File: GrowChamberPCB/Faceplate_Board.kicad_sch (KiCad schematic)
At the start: 4 parts, among them J10 Conn_01x24_Pin, J6 Conn_01x04_Pin

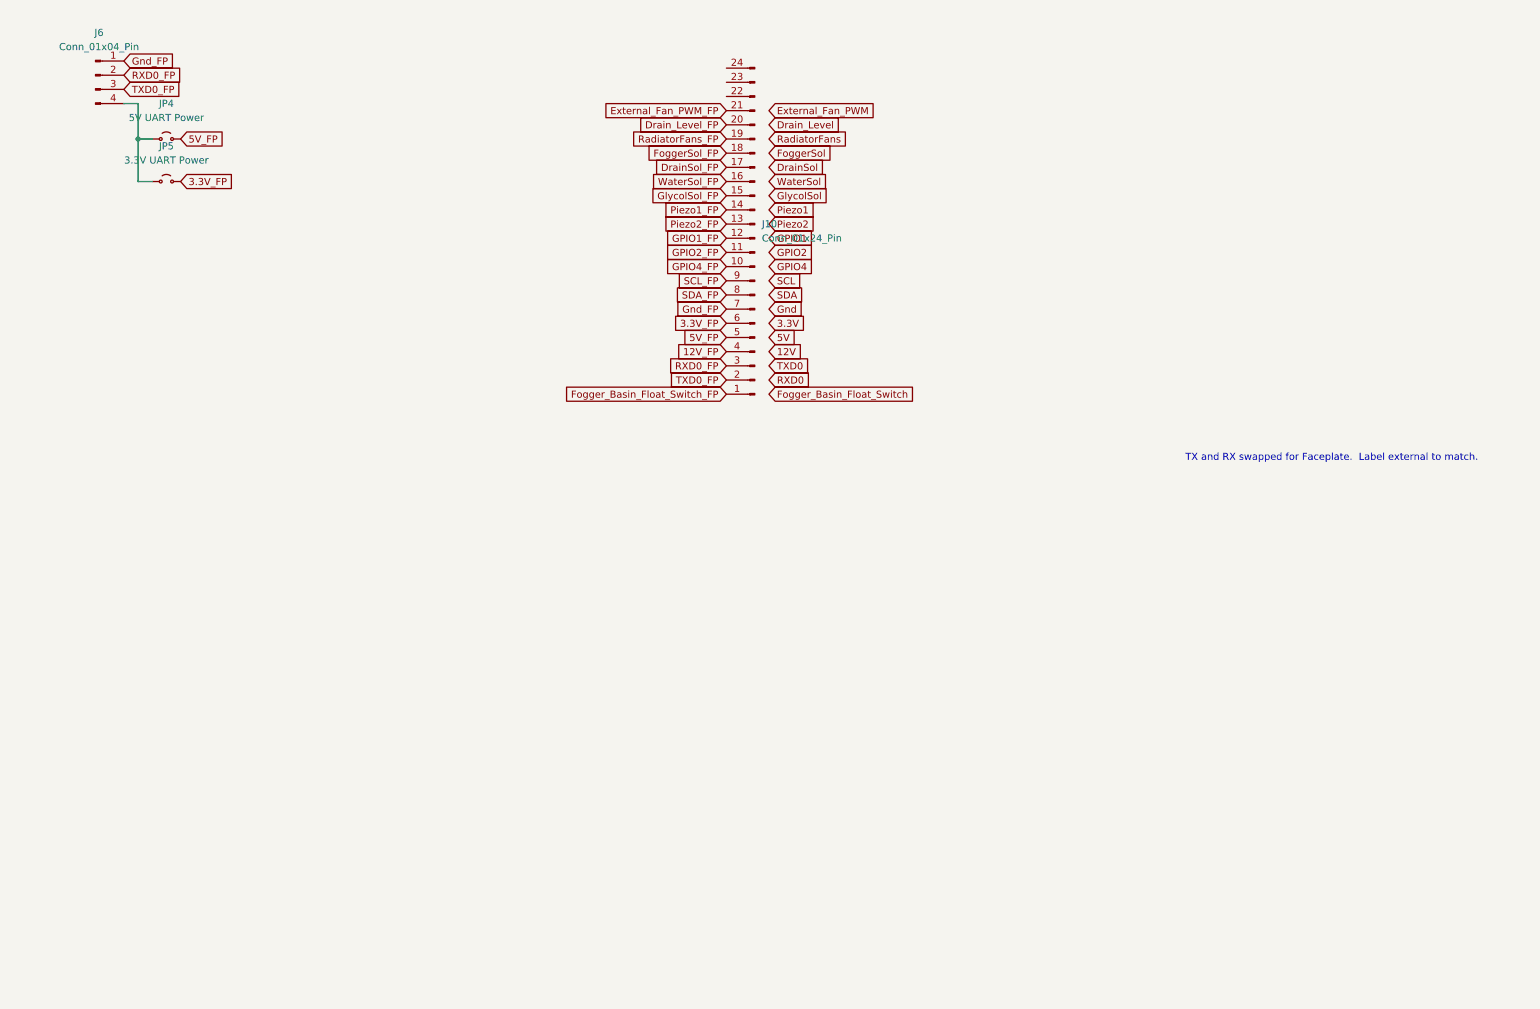
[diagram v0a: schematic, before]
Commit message: Working on faceplate
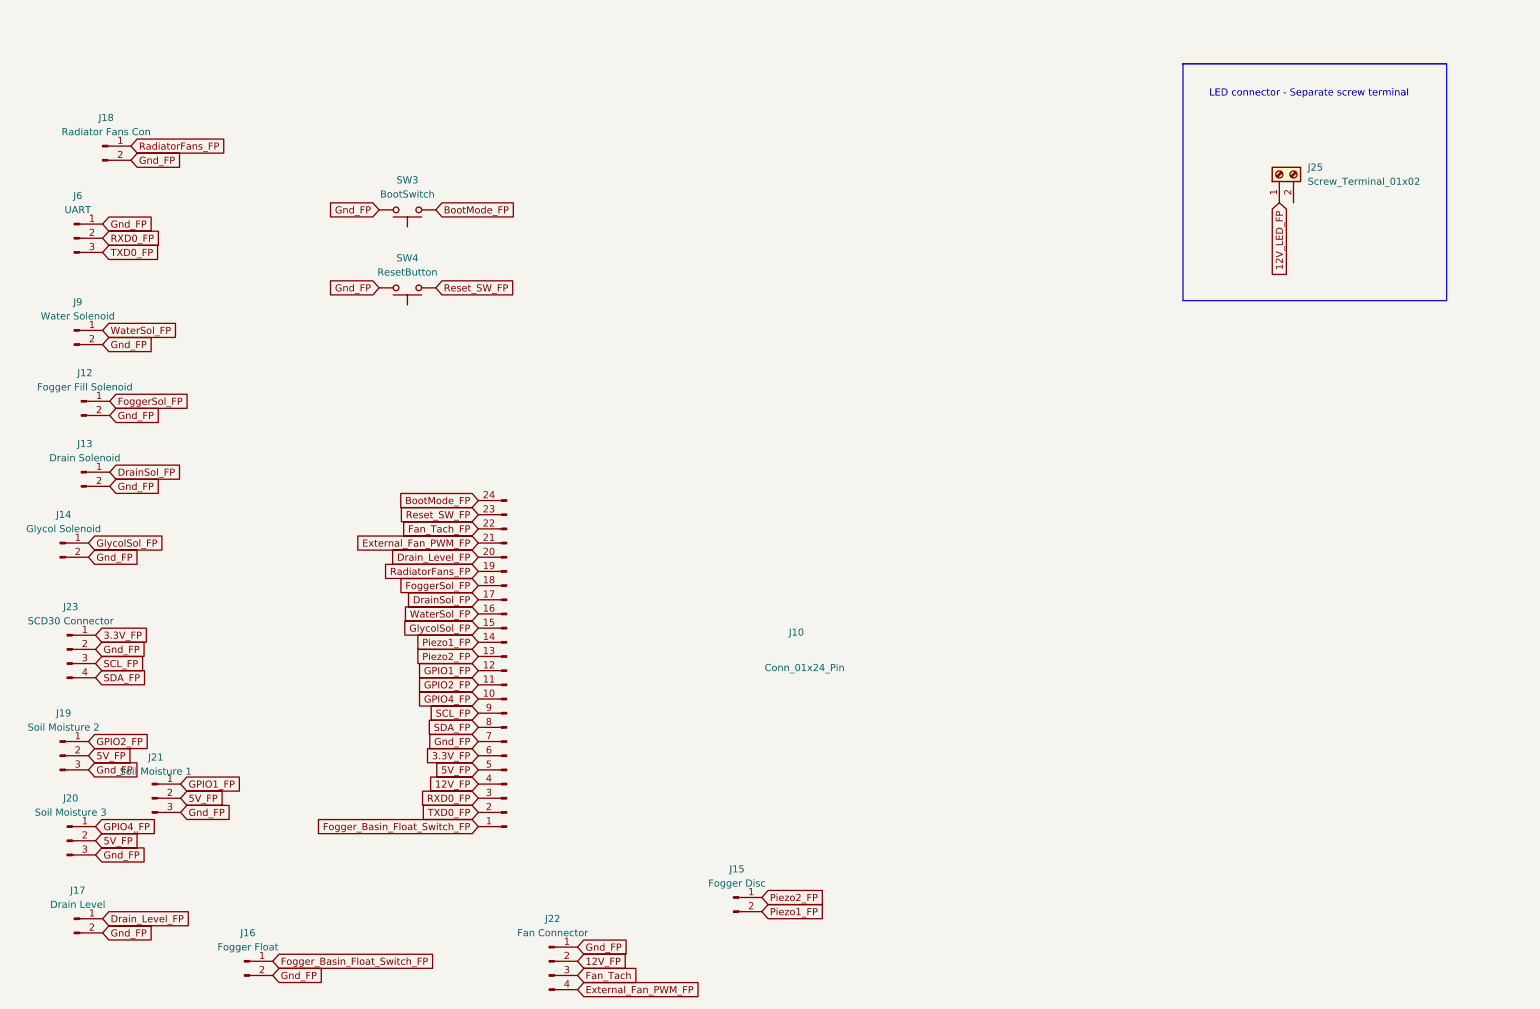
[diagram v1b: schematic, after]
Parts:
- removed J6: Conn_01x04_Pin, symbol Connector:Conn_01x04_Pin
- removed JP4: 5V UART Power, symbol Jumper:Jumper_2_Small_Open
- removed JP5: 3.3V UART Power, symbol Jumper:Jumper_2_Small_Open
- added J12: Fogger Fill Solenoid, symbol Connector:Conn_01x02_Pin
- added J13: Drain Solenoid, symbol Connector:Conn_01x02_Pin
- added J14: Glycol Solenoid, symbol Connector:Conn_01x02_Pin
- added J15: Fogger Disc, symbol Connector:Conn_01x02_Pin
- added J16: Fogger Float, symbol Connector:Conn_01x02_Pin
- added J17: Drain Level, symbol Connector:Conn_01x02_Pin
- added J18: Radiator Fans Con, symbol Connector:Conn_01x02_Pin
- added J19: Soil Moisture 2, Connector_Molex:Molex_KK-254_AE-6410-03A_1x03_P2.54mm_Vertical, symbol Connector:Conn_01x03_Pin
- added J20: Soil Moisture 3, Connector_Molex:Molex_KK-254_AE-6410-03A_1x03_P2.54mm_Vertical, symbol Connector:Conn_01x03_Pin
- added J21: Soil Moisture 1, Connector_Molex:Molex_KK-254_AE-6410-03A_1x03_P2.54mm_Vertical, symbol Connector:Conn_01x03_Pin
- added J22: Fan Connector, symbol Connector:Conn_01x04_Pin
- added J23: SCD30 Connector, symbol Connector:Conn_01x04_Pin
- added J25: Screw_Terminal_01x02, symbol Connector:Screw_Terminal_01x02
- added J6: UART, Connector_Molex:Molex_KK-254_AE-6410-03A_1x03_P2.54mm_Vertical, symbol Connector:Conn_01x03_Pin
- added J9: Water Solenoid, symbol Connector:Conn_01x02_Pin
- added SW3: BootSwitch, symbol Switch:SW_Push
- added SW4: ResetButton, symbol Switch:SW_Push
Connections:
- net 12V_FP: now also J22.2 (Pin_2)
- net 3.3V_FP: now also J23.1 (Pin_1)
- net 5V_FP: now also J19.2 (Pin_2), J20.2 (Pin_2), J21.2 (Pin_2)
- net DrainSol_FP: now also J13.1 (Pin_1)
- net Drain_Level_FP: now also J17.1 (Pin_1)
- net External_Fan_PWM_FP: now also J22.4 (Pin_4)
- net FoggerSol_FP: now also J12.1 (Pin_1)
- net Fogger_Basin_Float_Switch_FP: now also J16.1 (Pin_1)
- net GPIO1_FP: now also J21.1 (Pin_1)
- net GPIO2_FP: now also J19.1 (Pin_1)
- net GPIO4_FP: now also J20.1 (Pin_1)
- net GlycolSol_FP: now also J14.1 (Pin_1)
- net Gnd_FP: now also J12.2 (Pin_2), J13.2 (Pin_2), J14.2 (Pin_2), J16.2 (Pin_2), J17.2 (Pin_2), J18.2 (Pin_2), J19.3 (Pin_3), J20.3 (Pin_3), J21.3 (Pin_3), J22.1 (Pin_1), J23.2 (Pin_2), J6.1 (Pin_1), J9.2 (Pin_2), SW3.2, SW4.2
- net Piezo1_FP: now also J15.2 (Pin_2)
- net Piezo2_FP: now also J15.1 (Pin_1)
- net RXD0_FP: now also J6.2 (Pin_2)
- net RadiatorFans_FP: now also J18.1 (Pin_1)
- net SCL_FP: now also J23.3 (Pin_3)
- net SDA_FP: now also J23.4 (Pin_4)
- net TXD0_FP: now also J6.3 (Pin_3)
- net WaterSol_FP: now also J9.1 (Pin_1)
- net Fan_Tach_FP: now reaches J10.22 (Pin_22)
- net Reset_SW_FP: now reaches J10.23 (Pin_23)
- net Reset_SW_FP: now also SW4.1
- net BootMode_FP: now reaches J10.24 (Pin_24)
- net BootMode_FP: now also SW3.1
- new net 12V_LED_FP: J25.1 (Pin_1)
- new net Fan_Tach: J22.3 (Pin_3)
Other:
- note added: "LED connector - Separate screw terminal"
- note removed: "TX and RX swapped for Faceplate. Label external to match."
- moved on the sheet: J10

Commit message: final schematic
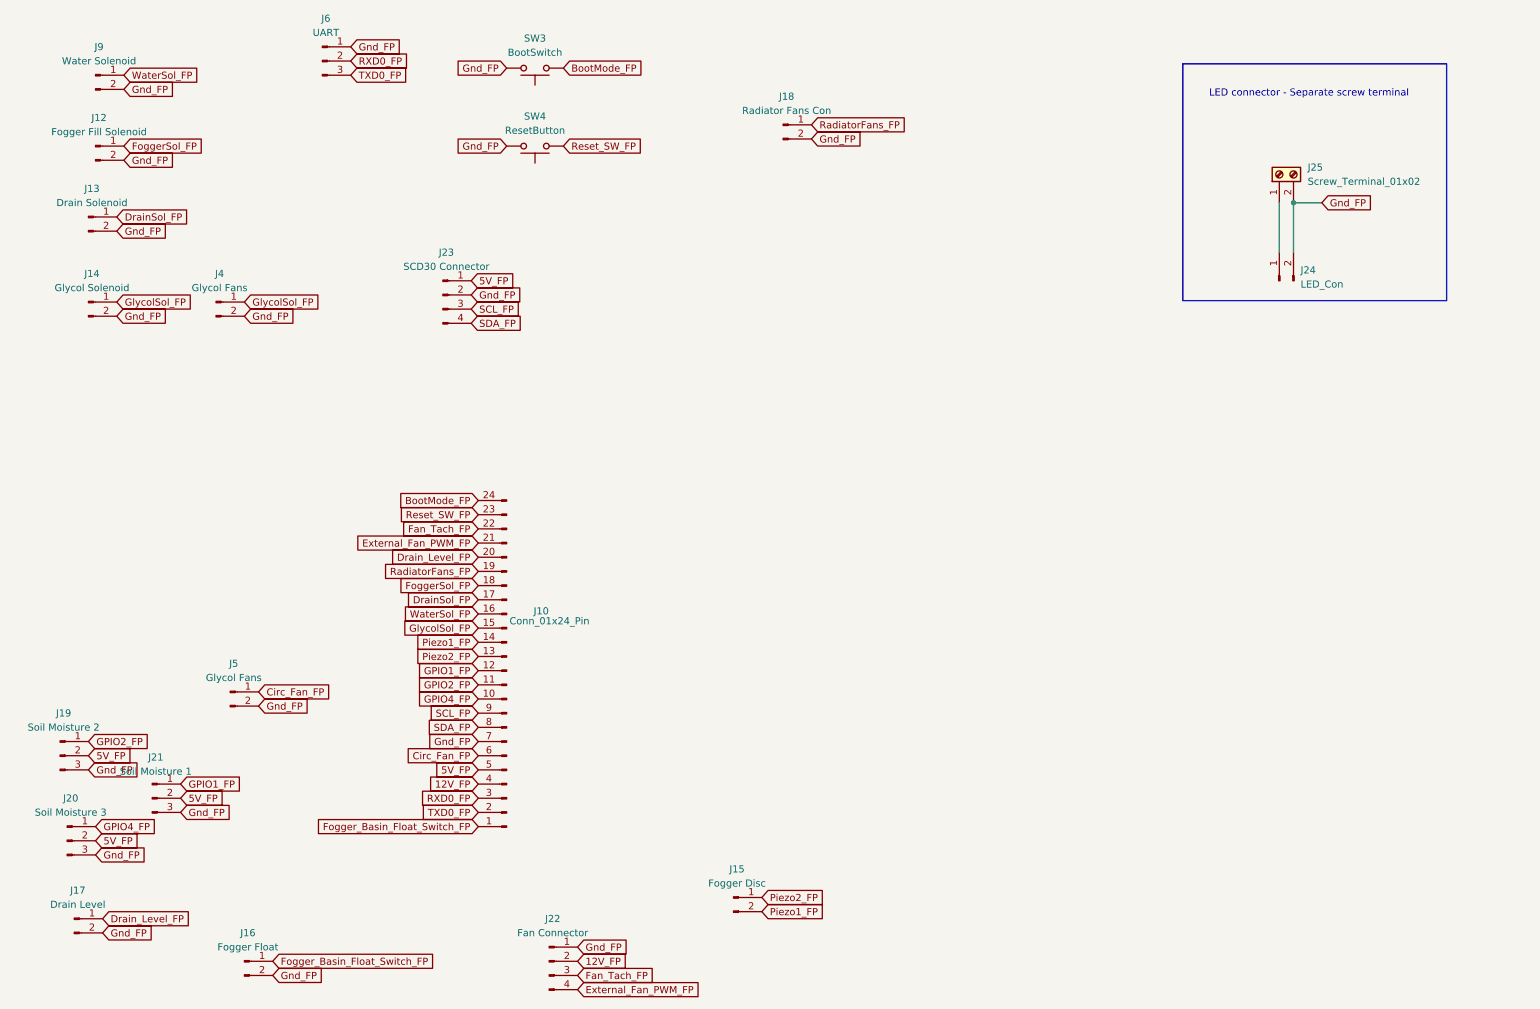
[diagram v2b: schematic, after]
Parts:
- added J24: LED_Con, symbol Connector:Conn_01x02_Pin
- added J4, J5: Glycol Fans, symbol Connector:Conn_01x02_Pin
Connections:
- net Fan_Tach is gone; now on net Fan_Tach_FP: J22.3 (Pin_3)
- net 5V_FP: now also J23.1 (Pin_1)
- net GlycolSol_FP: now also J4.1 (Pin_1)
- net Gnd_FP: now also J25.2 (Pin_2), J24.2 (Pin_2), J4.2 (Pin_2), J5.2 (Pin_2)
- net 12V_LED_FP: no longer names the net of J25.1 (Pin_1)
- net 12V_LED_FP: now also J24.1 (Pin_1)
- net 3.3V_FP renamed Circ_Fan_FP
- net Circ_Fan_FP: now also J5.1 (Pin_1); no longer J23.1 (Pin_1)
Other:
- moved on the sheet: J12, J13, J14, J18, J23, J6, J9, SW3, SW4
